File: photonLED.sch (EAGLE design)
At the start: 26 parts, among them IC1 7805DT, J1 3.5MM Screw Term, T1 MJD32C, T2 MJD32C, T3 MJD32C, T4 MJD32C, U3 TCS34725

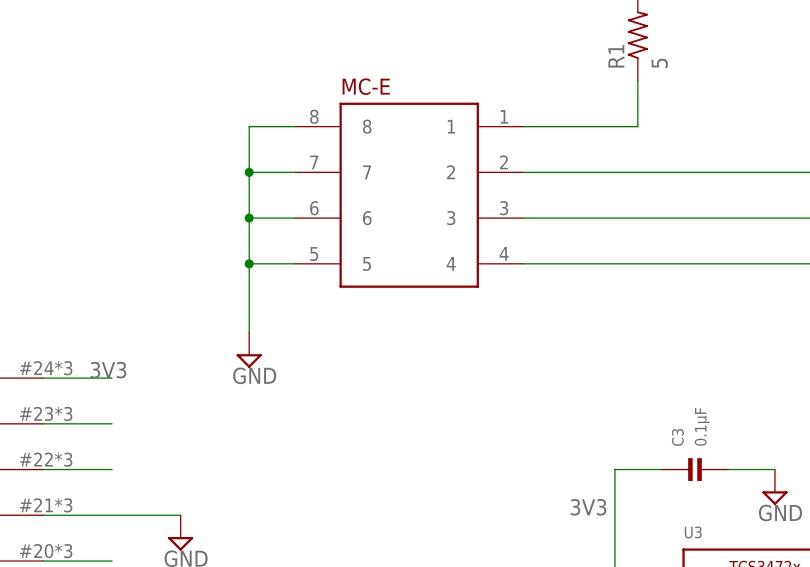
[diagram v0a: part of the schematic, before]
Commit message: final board layout
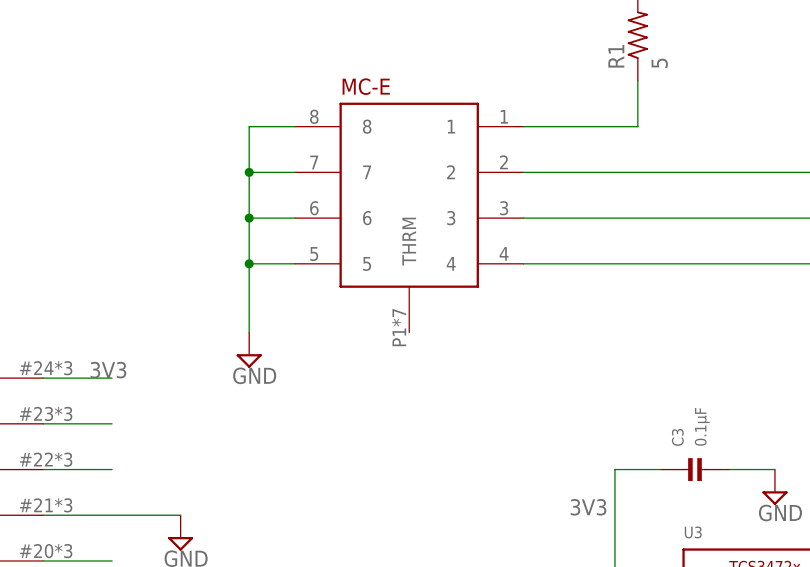
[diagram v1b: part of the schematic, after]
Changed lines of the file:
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@@
 <grid distance="0.1" unitdist="inch" unit="inch" style="lines" multiple="1" display="no" altdistance="0.01" altunitdist="inch" altunit="inch"/>
 <layers>
-<layer number="1" name="Top" color="4" fill="1" visible="yes" active="no"/>
-<layer number="2" name="Route2" color="1" fill="3" visible="yes" active="no"/>
-<layer number="3" name="Route3" color="4" fill="3" visible="yes" active="no"/>
-<layer number="14" name="Route14" color="1" fill="6" visible="yes" active="no"/>
-<layer number="15" name="Route15" color="4" fill="6" visible="yes" active="no"/>
-<layer number="16" name="Bottom" color="1" fill="1" visible="yes" active="no"/>
-<layer number="17" name="Pads" color="2" fill="1" visible="yes" active="no"/>
-<layer number="18" name="Vias" color="2" fill="1" visible="yes" active="no"/>
-<layer number="19" name="Unrouted" color="6" fill="1" visible="yes" active="no"/>
-<layer number="20" name="Dimension" color="15" fill="1" visible="yes" active="no"/>
-<layer number="21" name="tPlace" color="7" fill="1" visible="yes" active="no"/>
-<layer number="22" name="bPlace" color="7" fill="1" visible="yes" active="no"/>
-<layer number="23" name="tOrigins" color="15" fill="1" visible="yes" active="no"/>
-<layer number="24" name="bOrigins" color="15" fill="1" visible="yes" active="no"/>
-<layer number="25" name="tNames" color="7" fill="1" visible="yes" active="no"/>
-<layer number="26" name="bNames" color="7" fill="1" visible="yes" active="no"/>
-<layer number="27" name="tValues" color="7" fill="1" visible="yes" active="no"/>
-<layer number="28" name="bValues" color="7" fill="1" visible="yes" active="no"/>
+<layer number="1" name="Top" color="4" fill="1" visible="no" active="no"/>
+<layer number="2" name="Route2" color="1" fill="3" visible="no" active="no"/>
+<layer number="3" name="Route3" color="4" fill="3" visible="no" active="no"/>
+<layer number="14" name="Route14" color="1" fill="6" visible="no" active="no"/>
+<layer number="15" name="Route15" color="4" fill="6" visible="no" active="no"/>
+<layer number="16" name="Bottom" color="1" fill="1" visible="no" active="no"/>
+<layer number="17" name="Pads" color="2" fill="1" visible="no" active="no"/>
+<layer number="18" name="Vias" color="2" fill="1" visible="no" active="no"/>
+<layer number="19" name="Unrouted" color="6" fill="1" visible="no" active="no"/>
+<layer number="20" name="Dimension" color="15" fill="1" visible="no" active="no"/>
+<layer number="21" name="tPlace" color="7" fill="1" visible="no" active="no"/>
+<layer number="22" name="bPlace" color="7" fill="1" visible="no" active="no"/>
+<layer number="23" name="tOrigins" color="15" fill="1" visible="no" active="no"/>
+<layer number="24" name="bOrigins" color="15" fill="1" visible="no" active="no"/>
+<layer number="25" name="tNames" color="7" fill="1" visible="no" active="no"/>
+<layer number="26" name="bNames" color="7" fill="1" visible="no" active="no"/>
+<layer number="27" name="tValues" color="7" fill="1" visible="no" active="no"/>
+<layer number="28" name="bValues" color="7" fill="1" visible="no" active="no"/>
 <layer number="29" name="tStop" color="7" fill="3" visible="no" active="no"/>
 <layer number="30" name="bStop" color="7" fill="6" visible="no" active="no"/>
@@
 <layer number="35" name="tGlue" color="7" fill="4" visible="no" active="no"/>
 <layer number="36" name="bGlue" color="7" fill="5" visible="no" active="no"/>
-<layer number="37" name="tTest" color="7" fill="1" visible="yes" active="no"/>
-<layer number="38" name="bTest" color="7" fill="1" visible="yes" active="no"/>
+<layer number="37" name="tTest" color="7" fill="1" visible="no" active="no"/>
+<layer number="38" name="bTest" color="7" fill="1" visible="no" active="no"/>
 <layer number="39" name="tKeepout" color="4" fill="11" visible="no" active="no"/>
 <layer number="40" name="bKeepout" color="1" fill="11" visible="no" active="no"/>
@@
 <layer number="44" name="Drills" color="7" fill="1" visible="no" active="no"/>
 <layer number="45" name="Holes" color="7" fill="1" visible="no" active="no"/>
-<layer number="46" name="Milling" color="3" fill="1" visible="yes" active="no"/>
-<layer number="47" name="Measures" color="7" fill="1" visible="yes" active="no"/>
-<layer number="48" name="Document" color="7" fill="1" visible="yes" active="no"/>
-<layer number="49" name="Reference" color="7" fill="1" visible="yes" active="no"/>
-<layer number="50" name="dxf" color="7" fill="1" visible="yes" active="no"/>
-<layer number="51" name="tDocu" color="7" fill="1" visible="yes" active="no"/>
-<layer number="52" name="bDocu" color="7" fill="1" visible="yes" active="no"/>
-<layer number="53" name="tGND_GNDA" color="7" fill="9" visible="yes" active="no"/>
-<layer number="54" name="bGND_GNDA" color="1" fill="9" visible="yes" active="no"/>
-<layer number="56" name="wert" color="7" fill="1" visible="yes" active="no"/>
-<layer number="57" name="tCAD" color="7" fill="1" visible="yes" active="no"/>
-<layer number="59" name="tCarbon" color="7" fill="1" visible="yes" active="no"/>
-<layer number="60" name="bCarbon" color="7" fill="1" visible="yes" active="no"/>
+<layer number="46" name="Milling" color="3" fill="1" visible="no" active="no"/>
+<layer number="47" name="Measures" color="7" fill="1" visible="no" active="no"/>
+<layer number="48" name="Document" color="7" fill="1" visible="no" active="no"/>
+<layer number="49" name="Reference" color="7" fill="1" visible="no" active="no"/>
+<layer number="50" name="dxf" color="7" fill="1" visible="no" active="no"/>
+<layer number="51" name="tDocu" color="7" fill="1" visible="no" active="no"/>
+<layer number="52" name="bDocu" color="7" fill="1" visible="no" active="no"/>
+<layer number="53" name="tGND_GNDA" color="7" fill="9" visible="no" active="no"/>
+<layer number="54" name="bGND_GNDA" color="1" fill="9" visible="no" active="no"/>
+<layer number="56" name="wert" color="7" fill="1" visible="no" active="no"/>
+<layer number="57" name="tCAD" color="7" fill="1" visible="no" active="no"/>
+<layer number="59" name="tCarbon" color="7" fill="1" visible="no" active="no"/>
+<layer number="60" name="bCarbon" color="7" fill="1" visible="no" active="no"/>
 <layer number="90" name="Modules" color="5" fill="1" visible="yes" active="yes"/>
 <layer number="91" name="Nets" color="2" fill="1" visible="yes" active="yes"/>

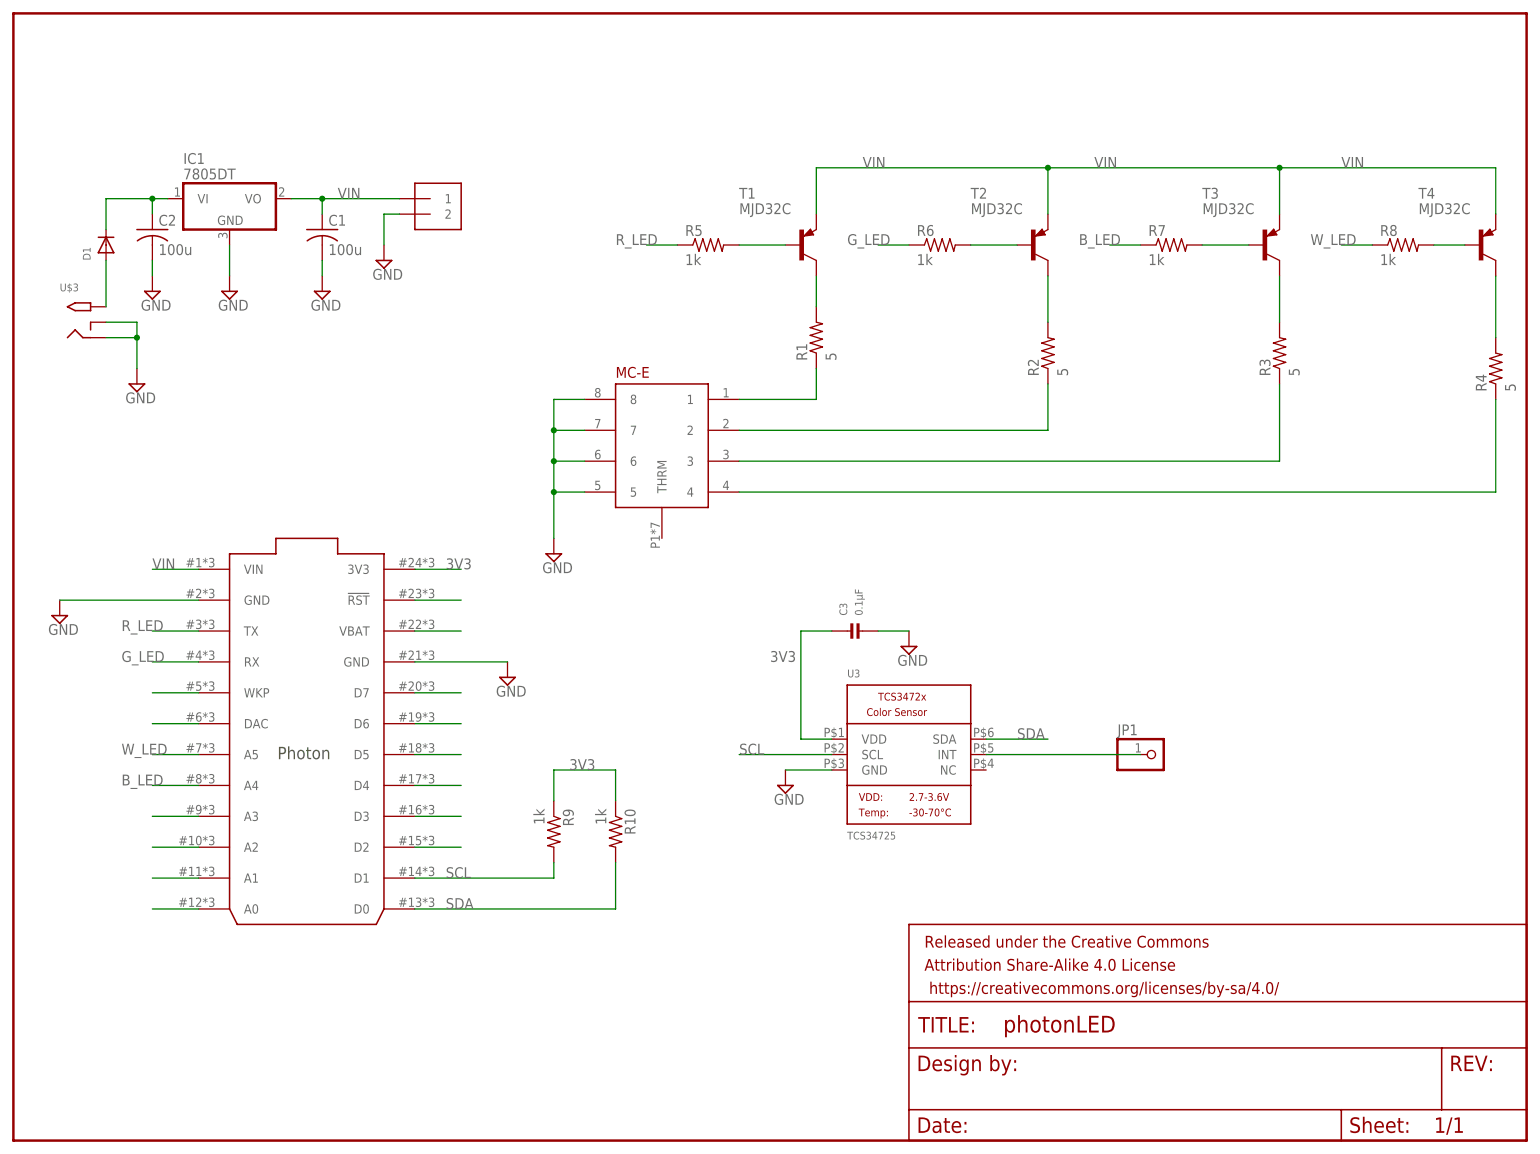
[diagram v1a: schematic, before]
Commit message: final board
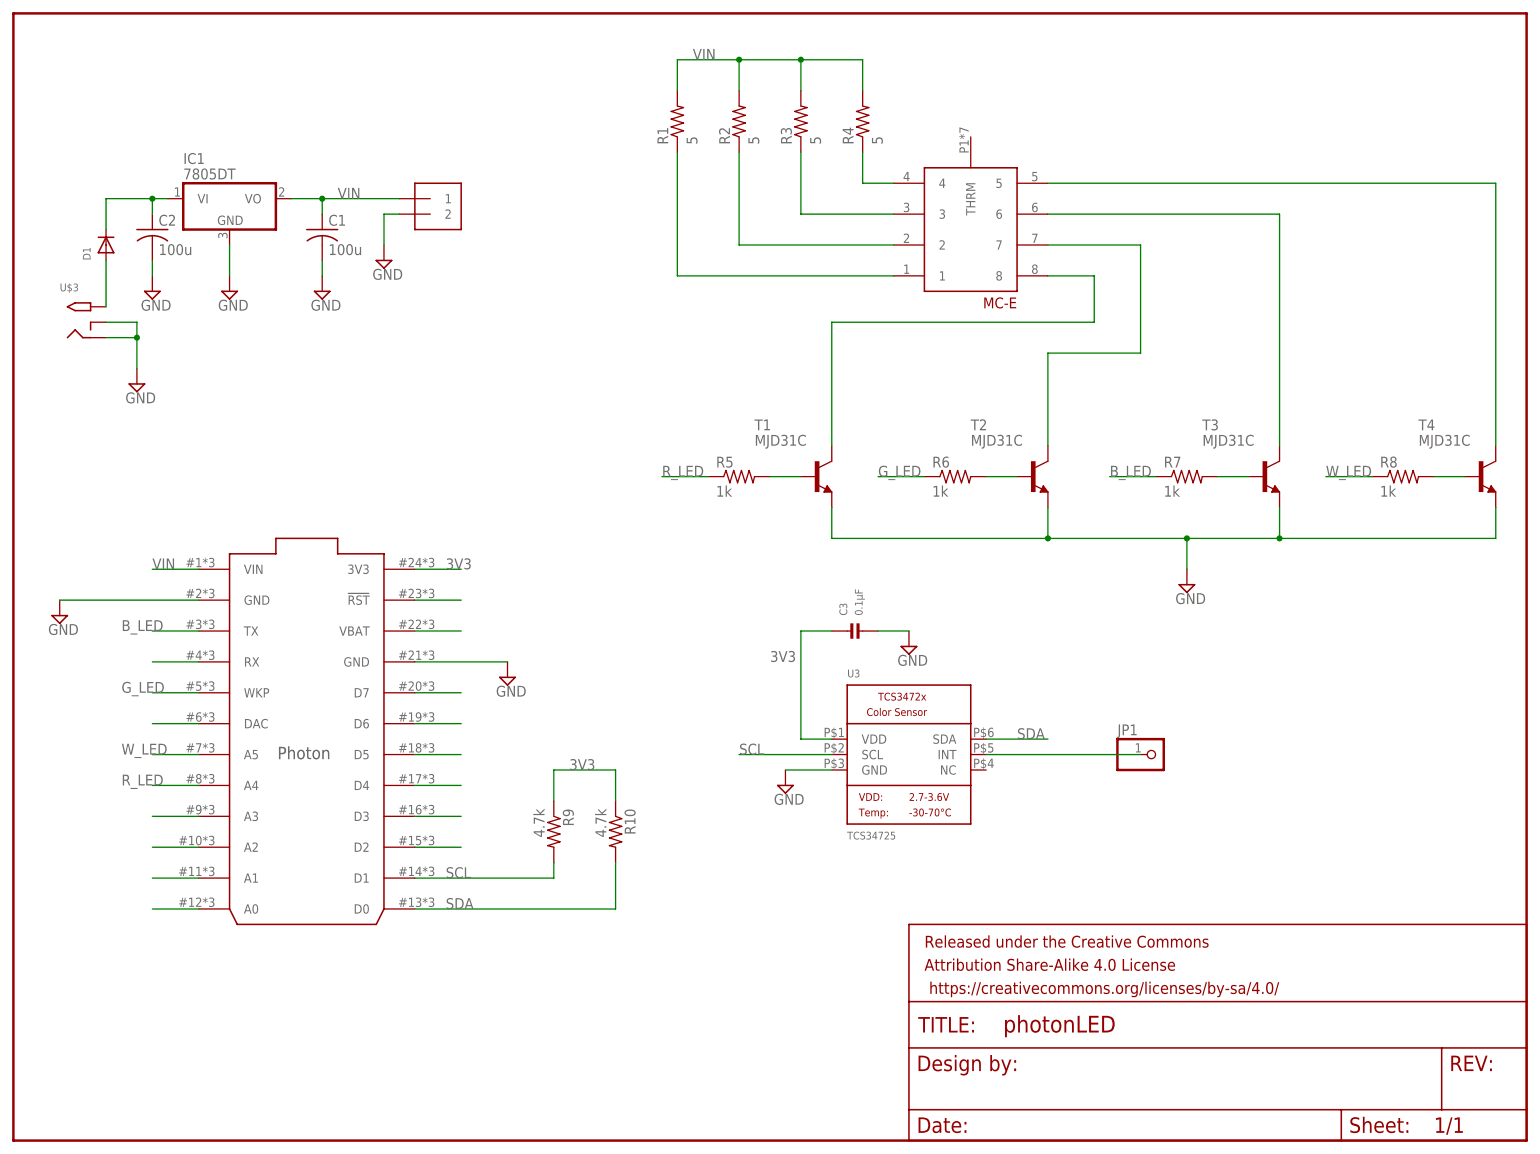
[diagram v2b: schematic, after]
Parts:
- R10, R9: value 1k -> 4.7k
- T1, T2, T3, T4: value MJD32C -> MJD31C; device transistor:MJD32C -> transistor:MJD31C
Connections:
- removed net N$13: U$1.WKP
- removed net N$6 (its old number): R2.2, T2.C
- new net N$15: U$1.RX
- new net N$18: T4.C, U$2.5
- net B_LED: now also U$1.TX; no longer U$1.A4
- net GND: now also T1.E, T2.E, T3.E, T4.E; no longer U$2.5, U$2.6, U$2.7, U$2.8
- net G_LED: now also U$1.WKP; no longer U$1.RX
- net N$5: now also U$2.8; no longer R1.2
- net N$7: now also T2.C, U$2.7; no longer R3.2, T3.C
- net N$8: now also T3.C, U$2.6; no longer R4.2, T4.C
- net R_LED: now also U$1.A4; no longer U$1.TX
- net VIN: now also R1.2, R2.2, R3.2, R4.2; no longer T1.E, T2.E, T3.E, T4.E
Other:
- moved on the sheet: R1, R2, R3, R4, R5, R6, R7, R8
